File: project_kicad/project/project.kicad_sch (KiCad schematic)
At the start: 19 parts

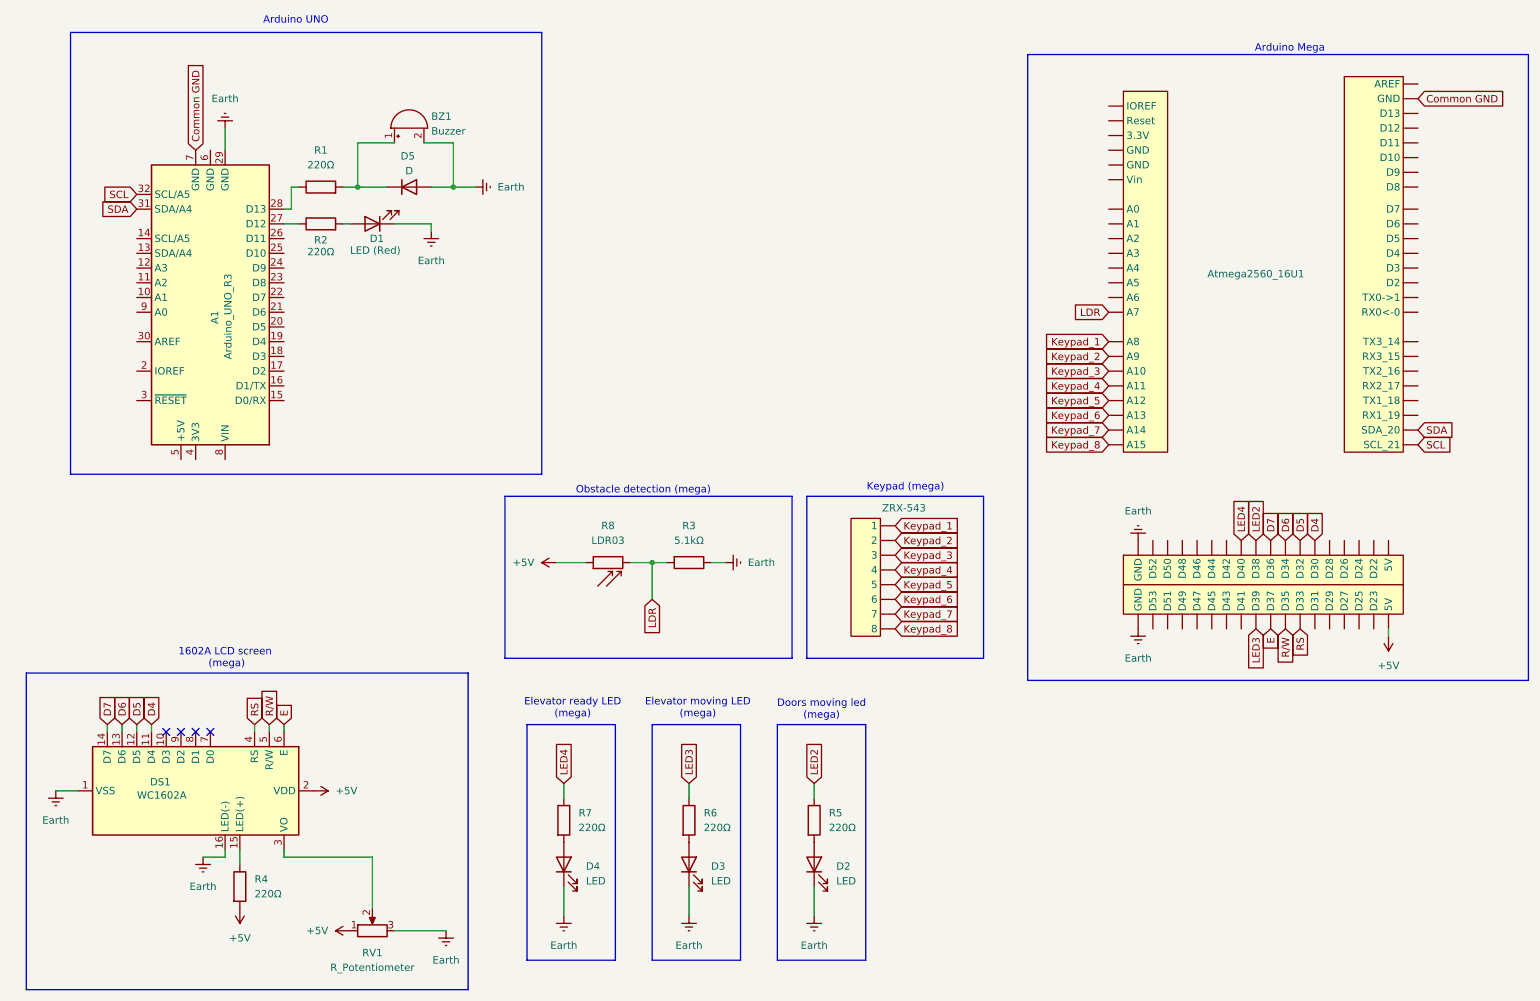
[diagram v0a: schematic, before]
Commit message: muokattu scematikki kuntoon
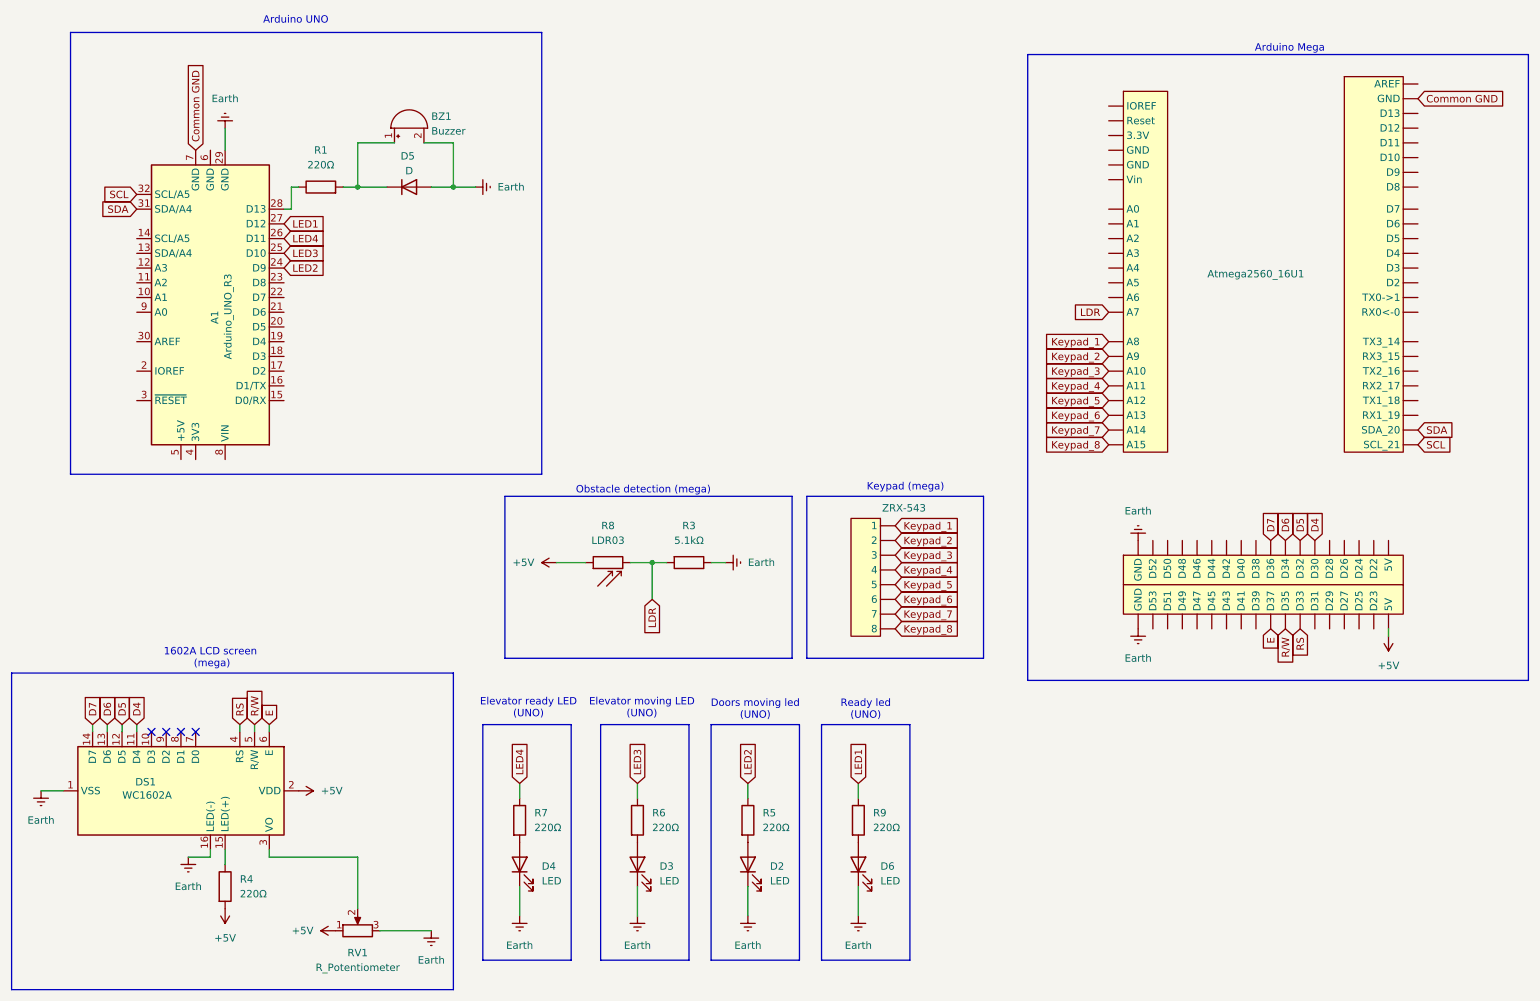
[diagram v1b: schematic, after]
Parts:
- removed D1: LED (Red), symbol Device:LED
- removed R2: 220Ω, symbol Device:R
- added D6: LED, symbol Device:LED
- added R9: 220Ω, symbol Device:R
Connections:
- net Earth: now also D6.1 (K)
- net LED2: now also A1.24 (D9); no longer Atmega2560_16U1. (SCL_21)
- net LED3: now also A1.25 (D10); no longer Atmega2560_16U1. (SCL_21)
- net LED4: now also A1.26 (D11); no longer Atmega2560_16U1. (SCL_21)
- net LED1: now reaches A1.27 (D12)
- net LED1: now also R9.1
- new net: D6.2 (A), R9.2
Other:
- note added: "Doors moving led (UNO)"
- note added: "Elevator moving LED (UNO)"
- note added: "Elevator ready LED (UNO)"
- note added: "Ready led (UNO)"
- note removed: "Doors moving led (mega)"
- note removed: "Elevator moving LED (mega)"
- note removed: "Elevator ready LED (mega)"
- moved on the sheet: D2, D3, D4, DS1, R4, R5, R6, R7, RV1
